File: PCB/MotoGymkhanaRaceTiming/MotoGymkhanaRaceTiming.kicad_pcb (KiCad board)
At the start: 2 copper layers, 116.8 x 64.8 mm, 31 parts, among them U1 LM2577T-ADJ_NOPB, U2 PC817, U3 PC817

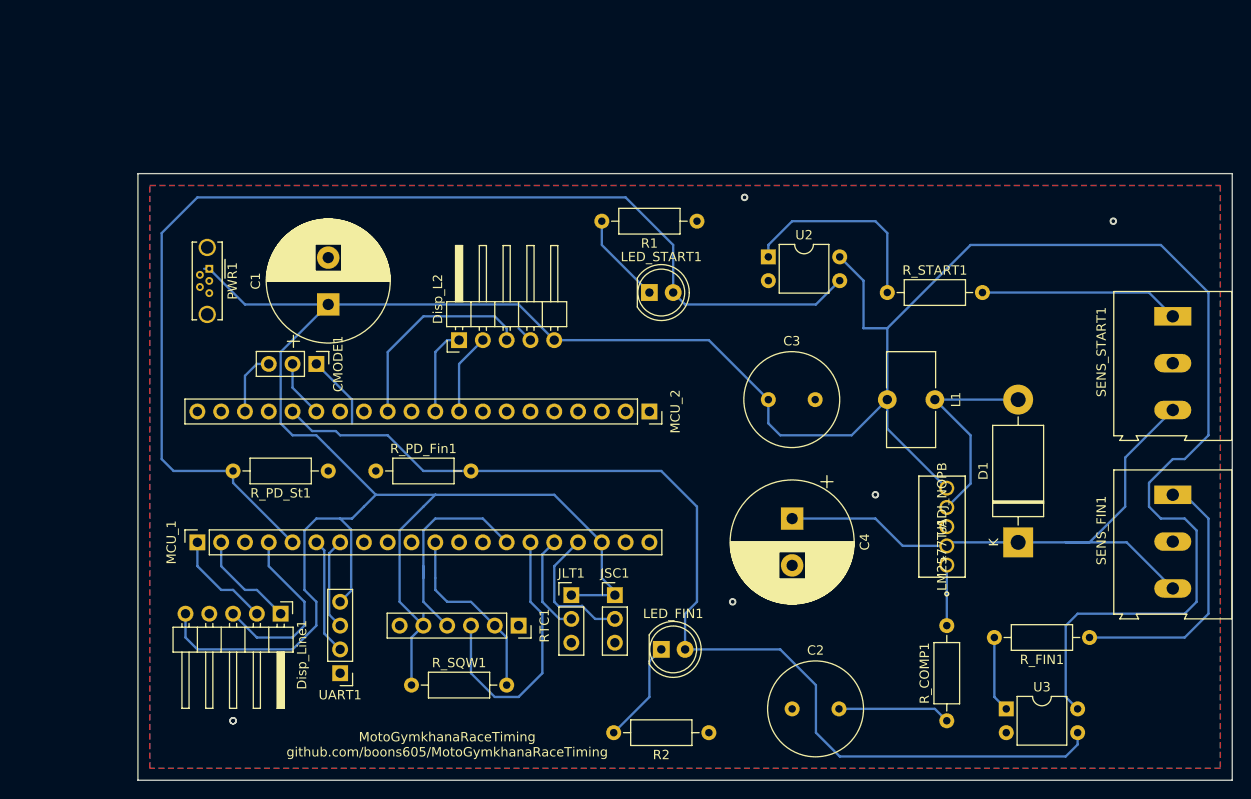
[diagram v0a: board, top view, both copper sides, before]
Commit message: PCB update
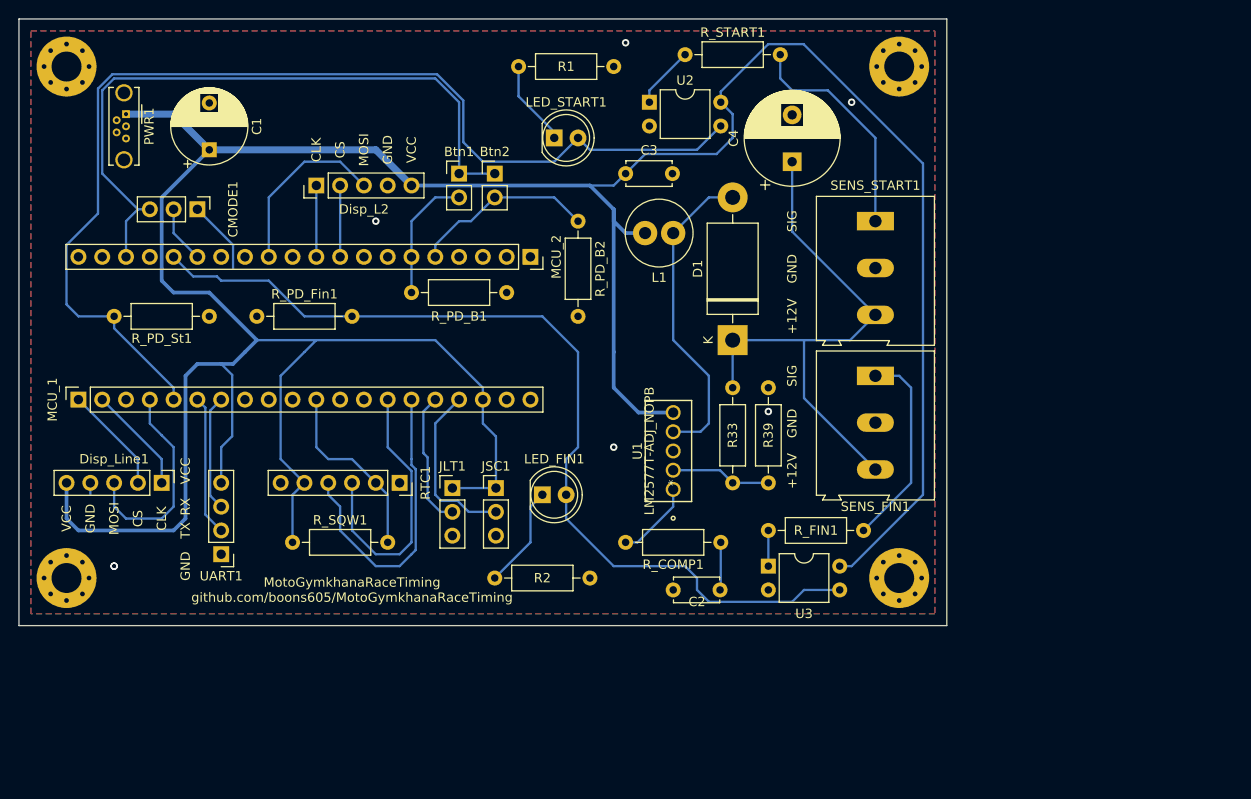
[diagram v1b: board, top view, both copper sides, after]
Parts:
- added Btn1: Conn_01x02_Male, Connector_PinHeader_2.54mm:PinHeader_1x02_P2.54mm_Vertical, F.Cu at (147.3, 76.2)
- added Btn2: Conn_01x02_Male, Connector_PinHeader_2.54mm:PinHeader_1x02_P2.54mm_Vertical, F.Cu at (151.1, 76.2)
- added H1: MountingHole_Pad, MountingHole:MountingHole_3.2mm_M3_Pad_Via, F.Cu at (194.3, 64.8)
- added H2: MountingHole_Pad, MountingHole:MountingHole_3.2mm_M3_Pad_Via, F.Cu at (194.3, 119.4)
- added H3: MountingHole_Pad, MountingHole:MountingHole_3.2mm_M3_Pad_Via, F.Cu at (105.4, 119.4)
- added H4: MountingHole_Pad, MountingHole:MountingHole_3.2mm_M3_Pad_Via, F.Cu at (105.4, 64.8)
- added R33: 33k, Resistor_THT:R_Axial_DIN0207_L6.3mm_D2.5mm_P10.16mm_Horizontal, F.Cu at (176.5, 109.2)
- added R39: 3k9, Resistor_THT:R_Axial_DIN0207_L6.3mm_D2.5mm_P10.16mm_Horizontal, F.Cu at (180.3, 99.1)
- added R_PD_B1: 10k, Resistor_THT:R_Axial_DIN0207_L6.3mm_D2.5mm_P10.16mm_Horizontal, F.Cu at (142.2, 88.9)
- added R_PD_B2: 10k, Resistor_THT:R_Axial_DIN0207_L6.3mm_D2.5mm_P10.16mm_Horizontal, F.Cu at (160.0, 81.3)
- C1: footprint Capacitor_THT:CP_Radial_D13.0mm_P5.00mm -> Capacitor_THT:CP_Radial_D8.0mm_P5.00mm
- C2, C3: footprint Capacitor_THT:C_Radial_D10.0mm_H12.5mm_P5.00mm -> Capacitor_THT:C_Disc_D4.7mm_W2.5mm_P5.00mm
- C4: footprint Capacitor_THT:CP_Radial_D13.0mm_P5.00mm -> Capacitor_THT:CP_Radial_D10.0mm_P5.00mm
- Disp_L2, Disp_Line1: footprint Connector_PinHeader_2.54mm:PinHeader_1x05_P2.54mm_Horizontal -> MotoGymkhanaRaceTiming:DisplayLineConnector
- L1: footprint Inductor_THT:L_Toroid_Vertical_L10.0mm_W5.0mm_P5.08mm -> Inductor_THT:L_Radial_D7.0mm_P3.00mm
- SENS_FIN1, SENS_START1: footprint TerminalBlock:TerminalBlock_Altech_AK300-3_P5.00mm -> MotoGymkhanaRaceTiming:SensorConnector
- U1: footprint footprints:LM2577T -> footprints:LM2577T-ADJ&slash_NOPB
- UART1: footprint Connector_PinHeader_2.54mm:PinHeader_1x04_P2.54mm_Vertical -> MotoGymkhanaRaceTiming:UART
- moved C4 38.1 mm to (182.9, 74.9), turned to 90 degrees
- moved D1 37.4 mm to (176.5, 94.0)
- moved SENS_FIN1 34.2 mm to (191.8, 97.8)
- moved R_START1 33.3 mm to (171.4, 63.5)
- moved SENS_START1 33.3 mm to (191.8, 81.3)
- moved L1 33.1 mm to (170.2, 82.5), turned to 180 degrees
- moved R_COMP1 30.7 mm to (175.3, 115.6), turned to 180 degrees
- moved U1 30.3 mm to (170.2, 109.2)
- moved U3 29.6 mm to (180.3, 118.1)
- moved C3 28.5 mm to (165.1, 76.2)
- moved R_FIN1 26.7 mm to (190.5, 114.3)
- moved Disp_L2 22.5 mm to (132.1, 77.5)
- moved U2 20.8 mm to (167.6, 68.6)
- moved R_PD_Fin1 20.8 mm to (125.7, 91.4)
- moved CMODE1 20.8 mm to (119.4, 80.0)
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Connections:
- RTC1 pad 3: Net-(MCU_1-Pad15) -> Net-(MCU_1-Pad14)
- RTC1 pad 4: Net-(MCU_1-Pad14) -> Net-(MCU_1-Pad15)
- U1 pad 2: Net-(C4-Pad1) -> Net-(R33-Pad1)
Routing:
- net Net-(Btn1-Pad1): track 6.88 -> 72.3 mm
- net Net-(Btn2-Pad2): track 0.00 -> 19.7 mm
- net Net-(C1-Pad1): track 356.7 -> 339.0 mm
- net Net-(R_START1-Pad1): track 21.9 -> 6.66 mm
- net Net-(LED_FIN1-Pad2): track 114.6 -> 99.9 mm
- net Net-(Btn1-Pad2): track 0.00 -> 13.8 mm
- net Net-(D1-Pad2): track 23.0 -> 35.3 mm
- net Net-(R33-Pad1): track 0.00 -> 10.7 mm
- net Net-(LED_START1-Pad2): track 125.4 -> 117.8 mm
- net Net-(R_FIN1-Pad1): track 28.8 -> 21.7 mm
- net Net-(C2-Pad2): track 12.0 -> 5.11 mm
- net Net-(MCU_1-Pad14): track 23.0 -> 29.3 mm
- net Net-(C4-Pad1): track 64.4 -> 58.4 mm
- net Net-(R_FIN1-Pad2): track 8.15 -> 3.81 mm
- net Net-(JLT1-Pad2): track 10.7 -> 14.5 mm
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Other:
- board size 116.8 x 64.8 mm -> 99.1 x 64.8 mm
